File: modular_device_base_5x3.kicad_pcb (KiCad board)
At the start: 2 copper layers, 83.8 x 40.6 mm, 23 parts, among them P1 PWR_JACK_2.5x5.5_SMD_RA, P2 HEADER_01X03_SMD_RA, P3 HEADER_01X03_SMD_RA, P4 HEADER_01X03_SMD_RA, P5 BNC_DOUBLE_RA, P6 HEADER_01X02_SMD_RA, P7 HEADER_01X02_SMD_RA, SW1 KT_SWITCH

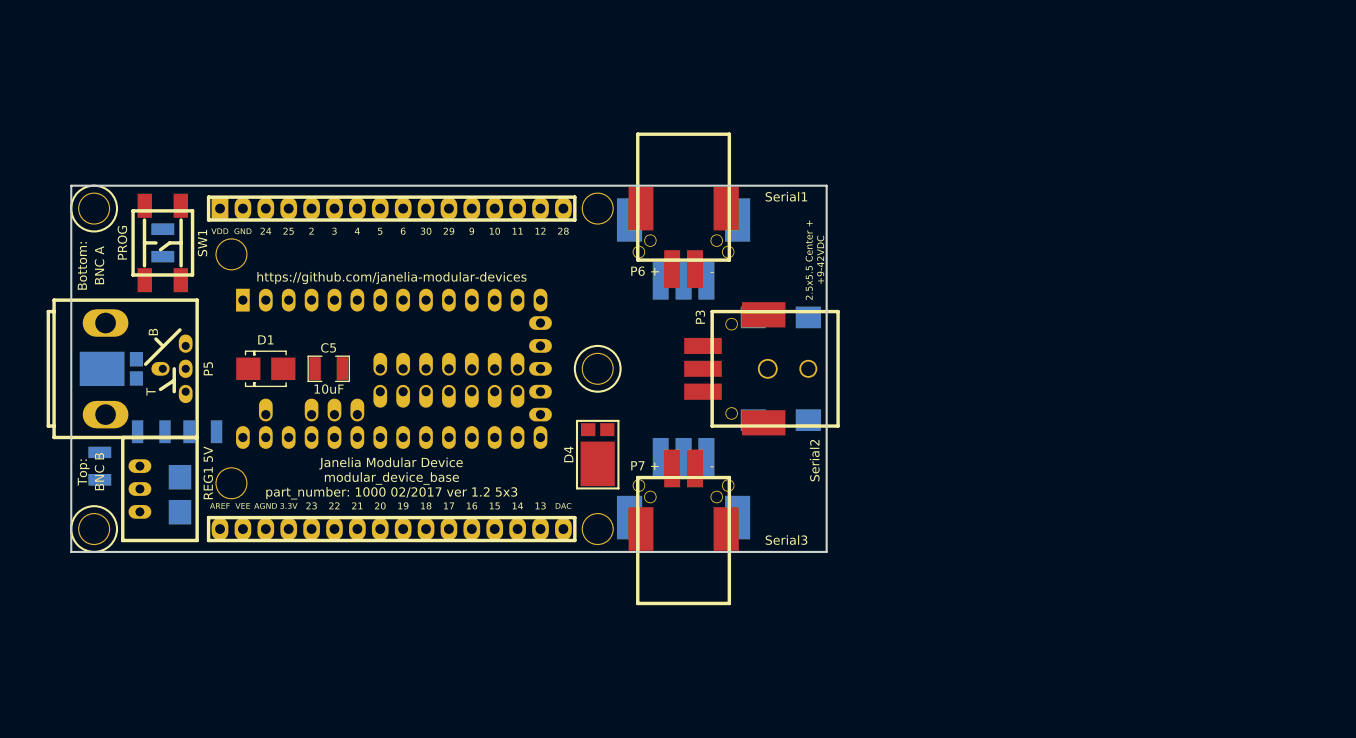
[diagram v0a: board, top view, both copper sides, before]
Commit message: Progress towards new modifications.
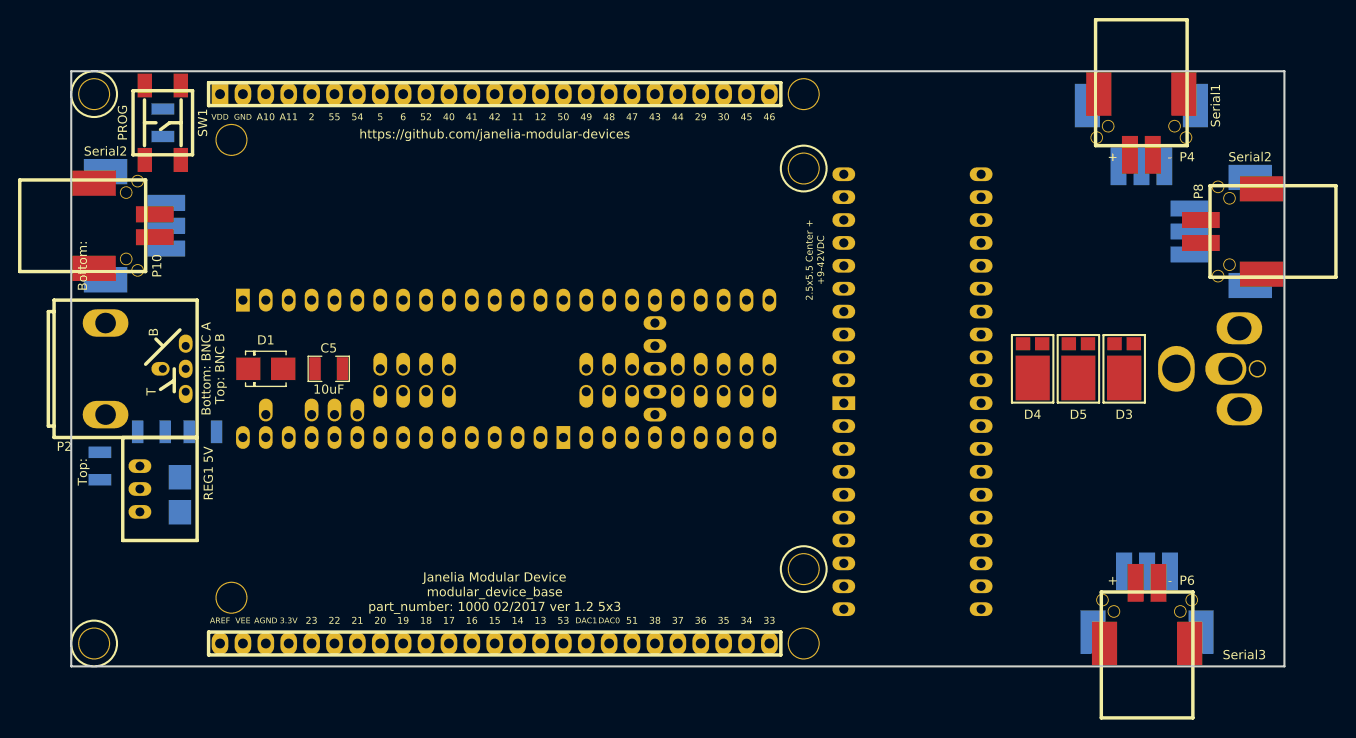
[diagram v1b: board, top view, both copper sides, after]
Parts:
- added D5: diode_schottky_45V_10A, modular_device_base_5x3:CFP15, F.Cu at (171.4, 99.7)
- added E1: TEENSY_ETHERNET, footprints:TEENSY_ETHERNET, B.Cu at (153.0, 84.5)
- added MH4: MNT_HOLE, modular_device_base_5x3:MOUNTING_HOLE_4-40, F.Cu at (141.0, 121.9)
- added P10: HEADER_01X02_SMD_RA, modular_device_base_5x3:Header_2_Pin_SMD_RA, F.Cu at (62.2, 83.8)
- added P8: HEADER_01X02_SMD_RA, modular_device_base_5x3:Header_2_Pin_SMD_RA, F.Cu at (191.8, 84.5)
- added P9: HEADER_01X03_SMD_RA, modular_device_base_5x3:Header_3_Pin_SMD_RA, B.Cu at (63.5, 83.8)
- D3: moved to F.Cu
- MDB1: value modular_device_base_5x3_FEMALE -> MODULAR_DEVICE_BASE_5x3_FEMALE; footprint modular_device_base_5x3:MODULAR_DEVICE_BASE_5X3_FEMALE -> footprints:MODULAR_DEVICE_BASE_5X3_FEMALE
- P1: value PWR_JACK_2.5x5.5_SMD_RA -> PWR_JACK_2.5x5.5; footprint modular_device_base_5x3:DCJACK_2PIN_HIGHCURRENT_SMD_RA -> footprints:DCJACK_2PIN_HIGHCURRENT
- P2: value HEADER_01X03_SMD_RA -> BNC_DOUBLE_RA; footprint modular_device_base_5x3:Header_3_Pin_SMD_RA -> modular_device_base_5x3:BNC_DOUBLE; moved to F.Cu
- P3: moved to B.Cu
- P4: value HEADER_01X03_SMD_RA -> HEADER_01X02_SMD_RA; footprint modular_device_base_5x3:Header_3_Pin_SMD_RA -> modular_device_base_5x3:Header_2_Pin_SMD_RA; moved to F.Cu
- P5: value BNC_DOUBLE_RA -> HEADER_01X03_SMD_RA; footprint modular_device_base_5x3:BNC_DOUBLE -> modular_device_base_5x3:Header_3_Pin_SMD_RA; moved to B.Cu
- P7: value HEADER_01X02_SMD_RA -> HEADER_01X03_SMD_RA; footprint modular_device_base_5x3:Header_2_Pin_SMD_RA -> modular_device_base_5x3:Header_3_Pin_SMD_RA; moved to B.Cu
- TEENSY1: value TEENSY_3_2 -> TEENSY_3.5; footprint modular_device_base_5x3:TEENSY_3.2 -> footprints:TEENSY_3.5
- moved P5 119.2 mm to (179.1, 128.9), turned to 0 degrees
- moved D3 112.4 mm to (176.5, 99.7), turned to 0 degrees
- moved P7 71.0 mm to (190.5, 84.5), turned to 90 degrees
- moved P6 70.5 mm to (179.1, 130.2), turned to 180 degrees
- moved P4 69.2 mm to (178.4, 69.2)
- moved P2 66.2 mm to (63.5, 99.7), turned to 90 degrees
- moved P1 55.9 mm to (194.3, 99.7), turned to 90 degrees
- moved P3 51.1 mm to (178.4, 70.5), turned to 180 degrees
- moved D4 49.2 mm to (166.4, 99.7)
- moved MH3 31.9 mm to (141.0, 77.5)
- moved C3 13.3 mm to (69.8, 72.4)
- moved SW1 13.3 mm to (69.8, 72.4)
- moved MH2 12.7 mm to (62.2, 130.2)
- moved MH1 12.7 mm to (62.2, 69.2)
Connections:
- P2 pad 1: /RX1 -> /BNC_A
- P2 pad 3: /TX1 -> /BNC_B
- P3 pad 1: /RX2 -> /RX1
- P3 pad 3: /TX2 -> /TX1
- P4 pad 1: /RX3 -> VCC
- P5 pad 1: /BNC_A -> /RX3
- P5 pad 3: /BNC_B -> /TX3
- P6 pad 1: VCC -> GND
- P6 pad 2: GND -> VDD
- P7 pad 1: GND -> /RX2
- P7 pad 2: VDD -> GND
- TEENSY1 pad 10: /D10 -> /TX2
- TEENSY1 pad 24: /D24 -> /E_CLK
- TEENSY1 pad 25: /D25 -> /E_RXER
- TEENSY1 pad 26: /RX2 -> /E_RXDV
- TEENSY1 pad 27: (no net) -> /E_TXEN
- TEENSY1 pad 28: /D28 -> /E_TXD0
- TEENSY1 pad 3: /D3 -> /E_RXD1
- TEENSY1 pad 31: /TX2 -> /RX4
- TEENSY1 pad 32: /BNC_B -> /TX4
- TEENSY1 pad 33: /BNC_A -> /D33
- TEENSY1 pad 4: /D4 -> /E_RXD0
- TEENSY1 pad 9: /D9 -> /RX2
- TEENSY1 pad A10: (no net) -> /A10
- TEENSY1 pad A11: (no net) -> /A11
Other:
- board size 83.8 x 40.6 mm -> 134.6 x 66 mm
